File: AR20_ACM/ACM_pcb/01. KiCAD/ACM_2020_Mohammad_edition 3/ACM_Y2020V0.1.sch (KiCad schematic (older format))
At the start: 32 parts, among them J1 TC2030-MCP-NL, P1 Conn_02x15_Odd_Even, Q1 Q_PMOS_DGS, U1 ATmega328P-AU, U2 MCP25625-x-SS, U3 NCV890430MW50TXG, Y1 16.0Mhz

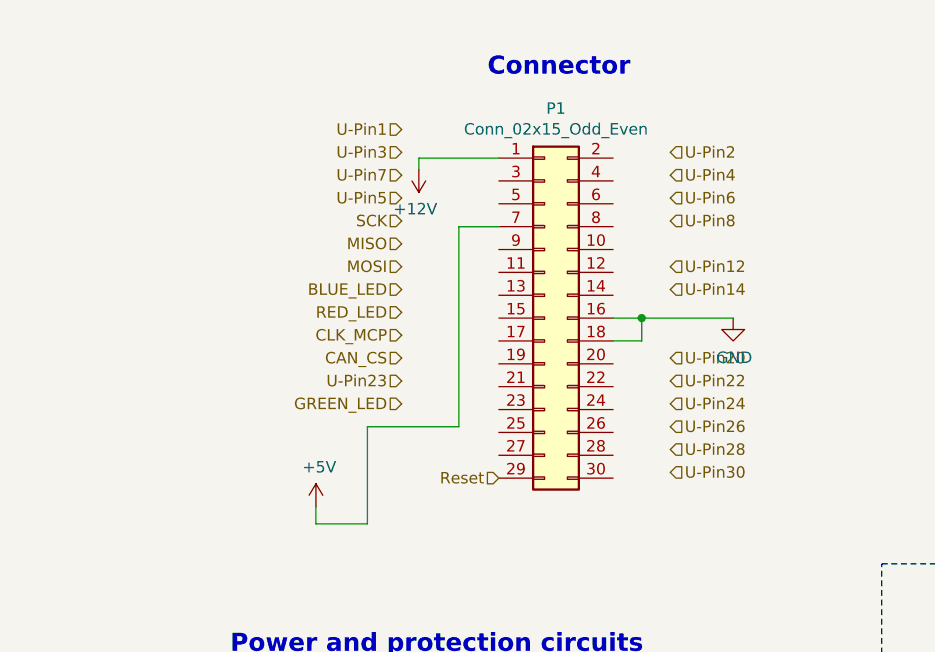
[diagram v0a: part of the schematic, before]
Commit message: ready pcb ACM
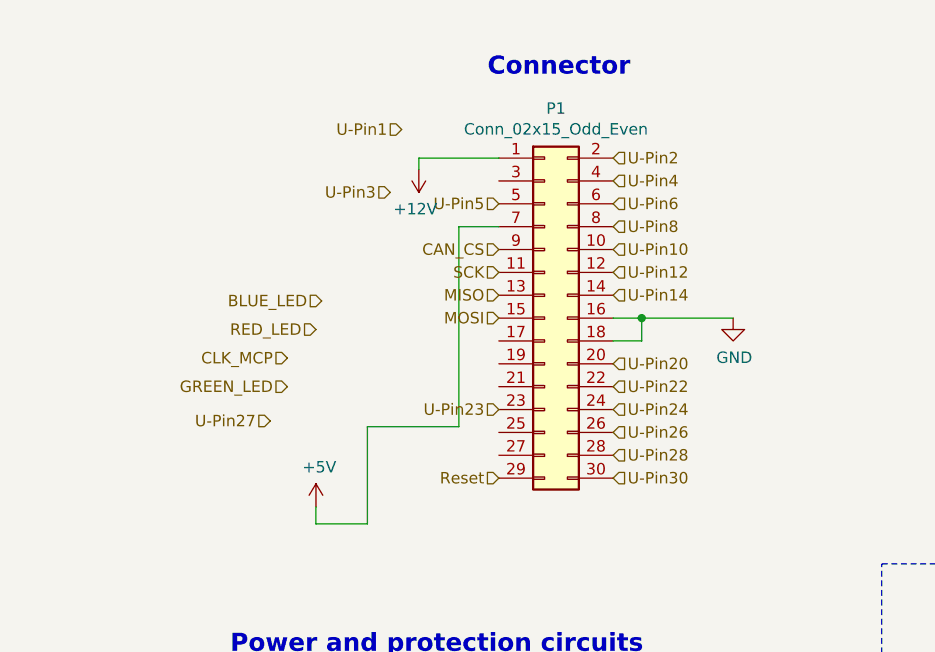
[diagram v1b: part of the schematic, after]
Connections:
- net CAN_CS: now also P1.9 (Pin_9)
- net MISO: now also P1.13 (Pin_13)
- net MOSI: now also P1.15 (Pin_15)
- net SCK: now also P1.11 (Pin_11)
- net U-Pin12: now also P1.12 (Pin_12)
- net U-Pin14: now also P1.14 (Pin_14)
- net U-Pin2: now also P1.2 (Pin_2)
- net U-Pin20: now also P1.20 (Pin_20)
- net U-Pin22: now also P1.22 (Pin_22)
- net U-Pin23: now also P1.23 (Pin_23)
- net U-Pin24: now also P1.24 (Pin_24)
- net U-Pin26: now also P1.26 (Pin_26)
- net U-Pin28: now also P1.28 (Pin_28)
- net U-Pin30: now also P1.30 (Pin_30)
- net U-Pin4: now also P1.4 (Pin_4)
- net U-Pin5: now also P1.5 (Pin_5)
- net U-Pin6: now also P1.6 (Pin_6)
- net U-Pin8: now also P1.8 (Pin_8)
- net U-Pin10: now reaches P1.10 (Pin_10)
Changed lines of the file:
@@
 Wire Wire Line
 	6725 1975 6725 1875
-Text HLabel 5675 1350 0    50   Input ~ 0
+Text HLabel 6100 1375 0    50   Input ~ 0
 U-Pin5
-Text HLabel 5675 1250 0    50   Input ~ 0
-U-Pin7
+Text HLabel 5100 2325 0    50   Input ~ 0
+U-Pin27
 Text HLabel 5675 1050 0    50   Input ~ 0
 U-Pin1
-Text HLabel 5675 1150 0    50   Input ~ 0
+Text HLabel 5625 1325 0    50   Input ~ 0
 U-Pin3
 Text HLabel 1575 6275 0    50   Input ~ 0
@@
 Wire Wire Line
 	3275 6075 3450 6075
-Text HLabel 5675 2250 0    50   Input ~ 0
+Text HLabel 5175 2175 0    50   Input ~ 0
 GREEN_LED
-Text HLabel 5675 2150 0    50   Input ~ 0
+Text HLabel 6100 2275 0    50   Input ~ 0
 U-Pin23
 $Comp
@@
 Wire Wire Line
 	6600 1875 6725 1875
-Text HLabel 6850 2350 2    50   Input ~ 0
+Text HLabel 6600 2375 2    50   Input ~ 0
 U-Pin26
-Text HLabel 6850 2450 2    50   Input ~ 0
+Text HLabel 6600 2475 2    50   Input ~ 0
 U-Pin28
-Text HLabel 6850 1450 2    50   Input ~ 0
+Text HLabel 6600 1475 2    50   Input ~ 0
 U-Pin8
 Text HLabel 6100 2575 0    50   Input ~ 0
@@
 Wire Wire Line
 	6725 1875 7125 1875
-Text HLabel 6850 1350 2    50   Input ~ 0
+Text HLabel 6600 1375 2    50   Input ~ 0
 U-Pin6
-Text HLabel 6850 2550 2    50   Input ~ 0
+Text HLabel 6600 2575 2    50   Input ~ 0
 U-Pin30
-Text HLabel 6850 2250 2    50   Input ~ 0
+Text HLabel 6600 2275 2    50   Input ~ 0
 U-Pin24
-Text HLabel 6850 2150 2    50   Input ~ 0
+Text HLabel 6600 2175 2    50   Input ~ 0
 U-Pin22
-Text HLabel 6850 2050 2    50   Input ~ 0
+Text HLabel 6600 2075 2    50   Input ~ 0
 U-Pin20
-Text HLabel 6850 1250 2    50   Input ~ 0
+Text HLabel 6600 1275 2    50   Input ~ 0
 U-Pin4
-Text HLabel 6850 1150 2    50   Input ~ 0
+Text HLabel 6600 1175 2    50   Input ~ 0
 U-Pin2
-Text HLabel 6850 1750 2    50   Input ~ 0
+Text HLabel 6600 1775 2    50   Input ~ 0
 U-Pin14
-Text HLabel 6850 1650 2    50   Input ~ 0
+Text HLabel 6600 1675 2    50   Input ~ 0
 U-Pin12
 $Comp
@@
 Wire Wire Line
 	5300 2775 5525 2775
-Text HLabel 5675 2050 0    50   Input ~ 0
+Text HLabel 6100 1575 0    50   Input ~ 0
 CAN_CS
-Text HLabel 5675 1950 0    50   Input ~ 0
+Text HLabel 5175 2050 0    50   Input ~ 0
 CLK_MCP
-Text HLabel 5675 1850 0    50   Input ~ 0
+Text HLabel 5300 1925 0    50   Input ~ 0
 RED_LED
-Text HLabel 5675 1750 0    50   Input ~ 0
+Text HLabel 5325 1800 0    50   Input ~ 0
 BLUE_LED
-Text HLabel 5675 1650 0    50   Input ~ 0
+Text HLabel 6100 1875 0    50   Input ~ 0
 MOSI
-Text HLabel 5675 1550 0    50   Input ~ 0
+Text HLabel 6100 1775 0    50   Input ~ 0
 MISO
-Text HLabel 5675 1450 0    50   Input ~ 0
+Text HLabel 6100 1675 0    50   Input ~ 0
 SCK
 Connection ~ 6725 1875
@@
 Wire Wire Line
 	6100 1175 5750 1175
+Text HLabel 6600 1575 2    50   Input ~ 0
+U-Pin10
 $EndSCHEMATC
